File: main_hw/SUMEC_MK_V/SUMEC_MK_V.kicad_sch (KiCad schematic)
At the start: 6 parts

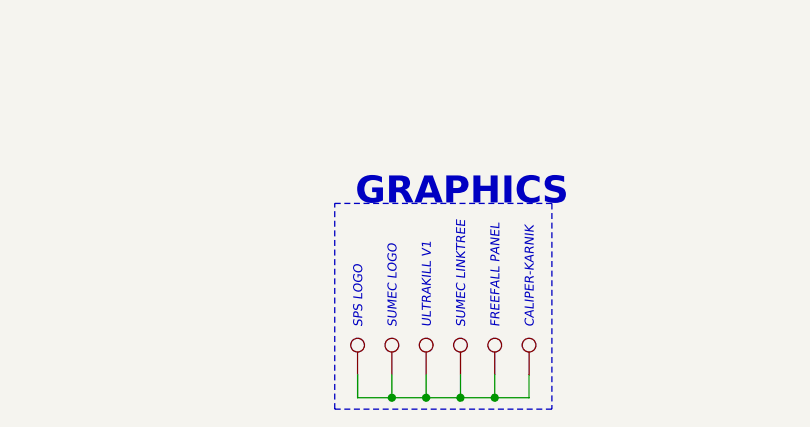
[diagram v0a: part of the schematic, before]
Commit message: new qre board
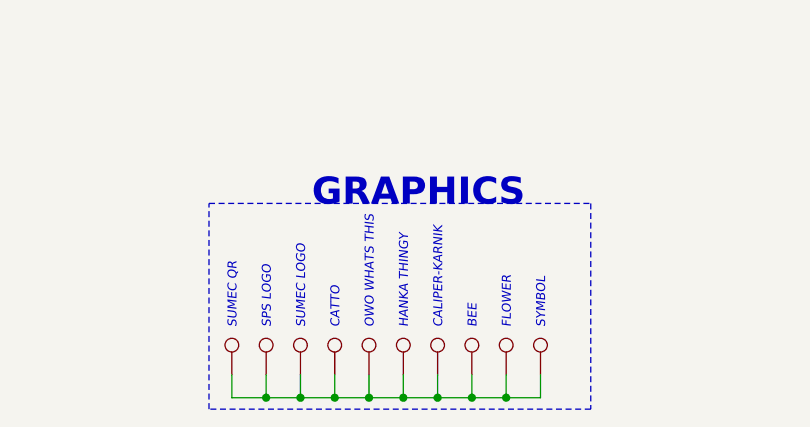
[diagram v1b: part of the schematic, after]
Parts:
- added TP19: TestPoint, sumec_graphic:SUMEC_QR_IMG, symbol Connector:TestPoint
- added TP20: TestPoint, sumec_graphic:BEE_IMG, symbol Connector:TestPoint
- added TP21: TestPoint, sumec_graphic:FLOWER_IMG, symbol Connector:TestPoint
- added TP22: TestPoint, sumec_graphic:SYMBOL_IMG, symbol Connector:TestPoint
- TP1: footprint (none) -> sumec_graphic:SPS_LOGO_IMG
- TP2: footprint (none) -> sumec_graphic:SUMEC_LOGO_IMG
- TP3: footprint (none) -> sumec_graphic:CATTO_MASK_IMG
- TP4: footprint (none) -> sumec_graphic:OWO_WHATS_THIS_IMG
- TP5: footprint (none) -> sumec_graphic:HANKA_THINGY_IMG
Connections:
- net at TP1.1, TP2.1, TP3.1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: now also TP19.1, TP20.1, TP21.1, TP22.1
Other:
- note added: "BEE"
- note added: "CATTO"
- note added: "FLOWER"
- note added: "HANKA THINGY"
- note added: "OWO WHATS THIS"
- note added: "SUMEC QR"
- note added: "SYMBOL"
- note removed: "FREEFALL PANEL"
- note removed: "SUMEC LINKTREE"
- note removed: "ULTRAKILL V1"
